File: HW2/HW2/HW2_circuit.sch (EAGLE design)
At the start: 23 parts, among them J2 LEFT, J3 RIGHT, X1 MINI-USB_SHIELD5P2-32005-601

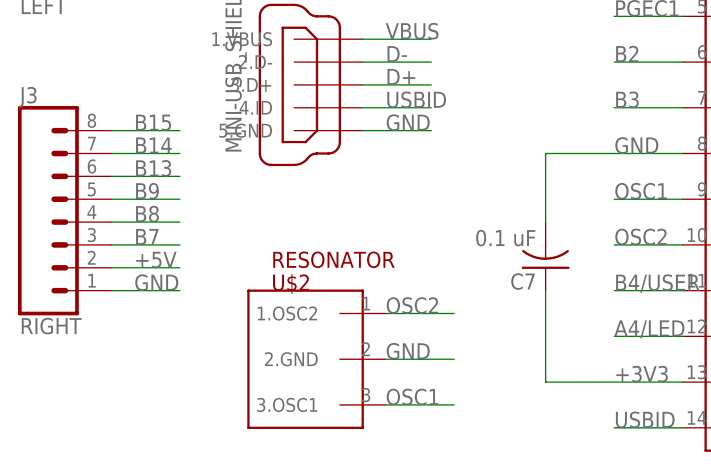
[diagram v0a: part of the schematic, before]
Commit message: Started Board Layout
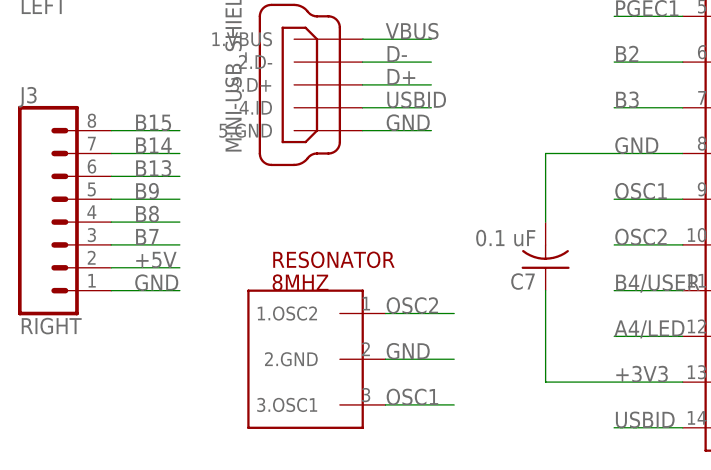
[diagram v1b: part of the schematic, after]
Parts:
- renumbered U$2 to 8MHZ
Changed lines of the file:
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@@
 <parts>
 <part name="U$1" library="ME433" deviceset="PIC32MX250F128B" device=""/>
-<part name="U$2" library="ME433" deviceset="RESONATOR" device=""/>
+<part name="8MHZ" library="ME433" deviceset="RESONATOR" device=""/>
 <part name="U$4" library="ME433" deviceset="MCP1702" device=""/>
 <part name="+3V1" library="ME433" deviceset="+3V3" device=""/>
@@
 <instances>
 <instance part="U$1" gate="G$1" x="35.56" y="5.08"/>
-<instance part="U$2" gate="G$1" x="-25.4" y="-20.32"/>
+<instance part="8MHZ" gate="G$1" x="-25.4" y="-20.32"/>
 <instance part="U$4" gate="G$1" x="101.6" y="53.34"/>
 <instance part="+3V1" gate="G$1" x="35.56" y="55.88"/>
@@
 </segment>
 <segment>
-<pinref part="U$2" gate="G$1" pin="2.GND"/>
+<pinref part="8MHZ" gate="G$1" pin="2.GND"/>
 <wire x1="-15.24" y1="-20.32" x2="-7.62" y2="-20.32" width="0.1524" layer="91"/>
 <label x="-15.24" y="-20.32" size="1.778" layer="95"/>
@@
 <net name="OSC2" class="0">
 <segment>
-<pinref part="U$2" gate="G$1" pin="1.OSC2"/>
+<pinref part="8MHZ" gate="G$1" pin="1.OSC2"/>
 <wire x1="-15.24" y1="-15.24" x2="-7.62" y2="-15.24" width="0.1524" layer="91"/>
 <label x="-15.24" y="-15.24" size="1.778" layer="95"/>
@@
 <net name="OSC1" class="0">
 <segment>
-<pinref part="U$2" gate="G$1" pin="3.OSC1"/>
+<pinref part="8MHZ" gate="G$1" pin="3.OSC1"/>
 <wire x1="-15.24" y1="-25.4" x2="-7.62" y2="-25.4" width="0.1524" layer="91"/>
 <label x="-15.24" y="-25.4" size="1.778" layer="95"/>
